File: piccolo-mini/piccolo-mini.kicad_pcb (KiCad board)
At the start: 2 copper layers, 96.1 x 20.6 mm, 16 parts, among them SW1 SW_Push, U1 ProMicro

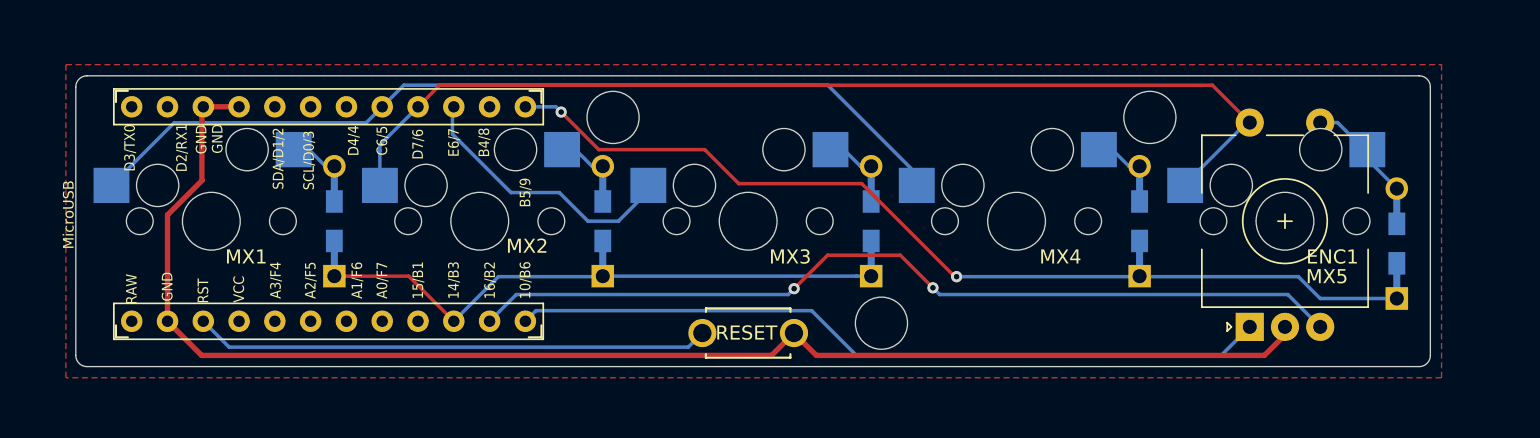
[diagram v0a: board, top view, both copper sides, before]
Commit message: Continued tweaks
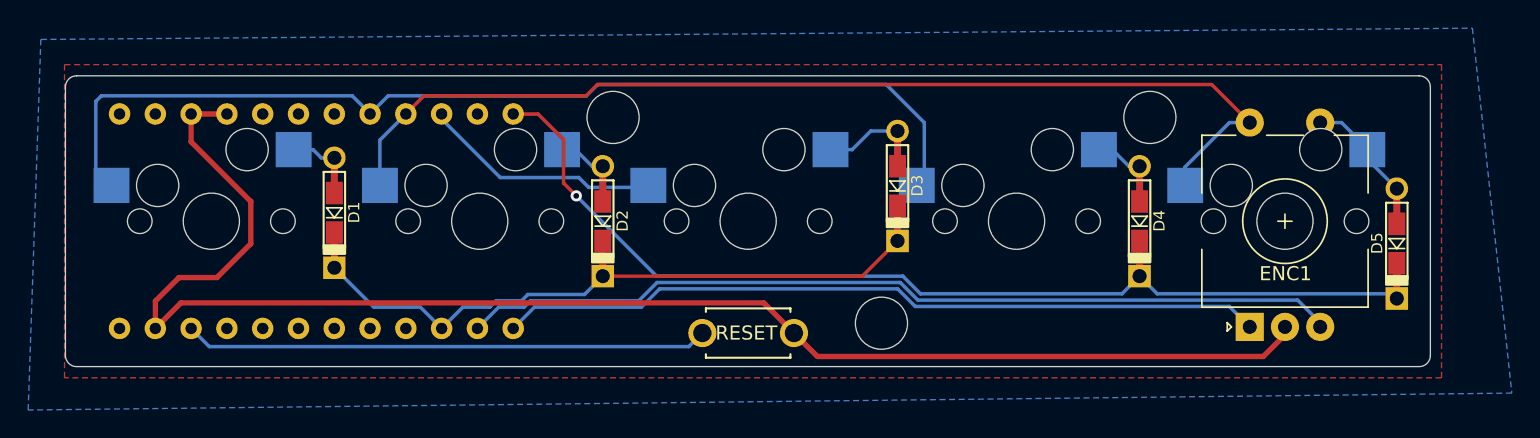
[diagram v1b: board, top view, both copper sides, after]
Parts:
- D1, D2, D3, D4, D5: footprint Keebio-Parts:Diode-Hybrid-Back -> Envoy:Diode-Hybrid-Back; moved to B.Cu
- MX1, MX2, MX3, MX4, MX5: footprint kbd:CherryMX_Hotswap -> Envoy:MXOnly-1U-Hotswap
- RESET1: renamed from SW1; footprint kbd:ResetSW -> Envoy:Reset_Jumper_Points
- U1: footprint Envoy:ProMicro_v3 -> Envoy:ProMicro_face_out; moved to B.Cu
- moved D3 3.12 mm to (192.4, 86.3)
- moved U1 1.00 mm to (151.7, 88.8), turned to -90 degrees
- moved D1 0.60 mm to (152.4, 88.2)
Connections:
- U1 pad 1: Net-(U1-Pad1) -> unconnected-(U1-Pad1)
- U1 pad 11: Net-(U1-Pad11) -> unconnected-(U1-Pad11)
- U1 pad 16: Net-(U1-Pad16) -> unconnected-(U1-Pad16)
- U1 pad 17: Net-(U1-Pad17) -> unconnected-(U1-Pad17)
- U1 pad 18: Net-(U1-Pad18) -> unconnected-(U1-Pad18)
- U1 pad 19: Net-(U1-Pad19) -> unconnected-(U1-Pad19)
- U1 pad 2: Net-(U1-Pad2) -> unconnected-(U1-Pad2)
- U1 pad 20: Net-(U1-Pad20) -> unconnected-(U1-Pad20)
- U1 pad 24: Net-(U1-Pad24) -> unconnected-(U1-Pad24)
- U1 pad 5: Net-(U1-Pad5) -> unconnected-(U1-Pad5)
- U1 pad 6: Net-(U1-Pad6) -> unconnected-(U1-Pad6)
- U1 pad 7: Net-(U1-Pad7) -> unconnected-(U1-Pad7)
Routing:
- net col0: track 63.5 -> 72.6 mm
- net GND: track 101.6 -> 107.7 mm
- net row0: track 40.8 -> 44.3 mm
- net row1: track 67.5 -> 70.9 mm, vias 2 -> 1
- net col2: track 19.2 -> 17.1 mm
- net Net-(D3-Pad2): track 3.38 -> 5.30 mm
- net col1: track 73.9 -> 74.9 mm
- net EncoderA: track 53.9 -> 54.6 mm
- net Reset: track 36.6 -> 37.2 mm
- net EncoderB: track 63.0 -> 62.6 mm, vias 2 -> 0
- added copper zone on B.Cu, net GND
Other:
- board size 96.1 x 20.6 mm -> 96.9 x 20.6 mm
- net class Default removed
- net class Power removed
